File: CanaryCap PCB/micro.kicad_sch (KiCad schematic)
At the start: 36 parts, among them SW1 SW_MEC_5E, SW2 SW_MEC_5E, SW4 SW_MEC_5E, U3 ESP32-C6FH4

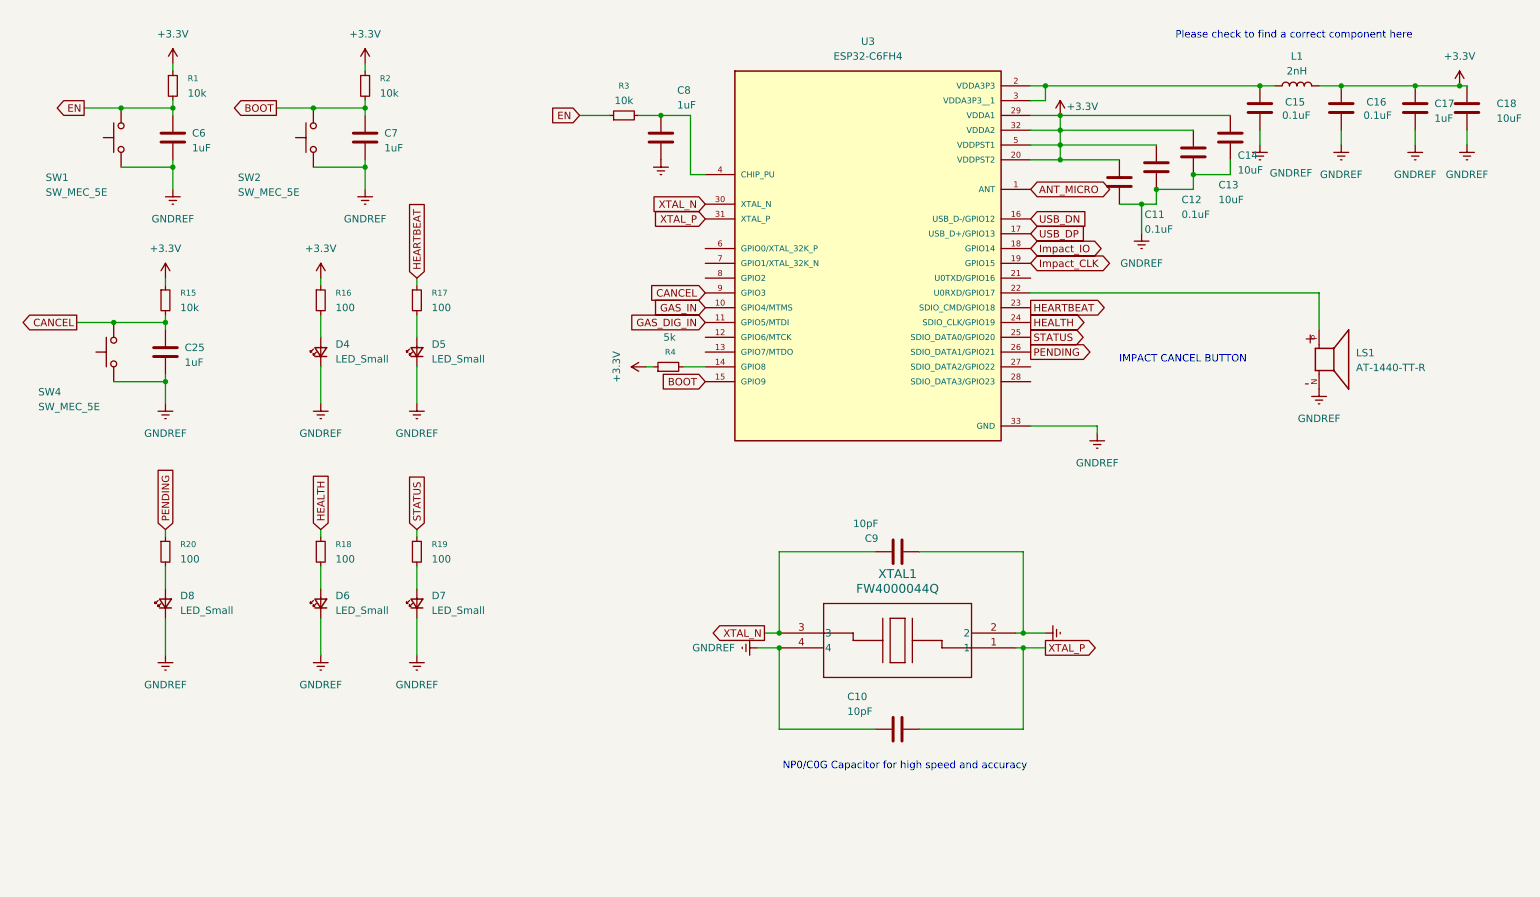
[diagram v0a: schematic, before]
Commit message: YIPPEE
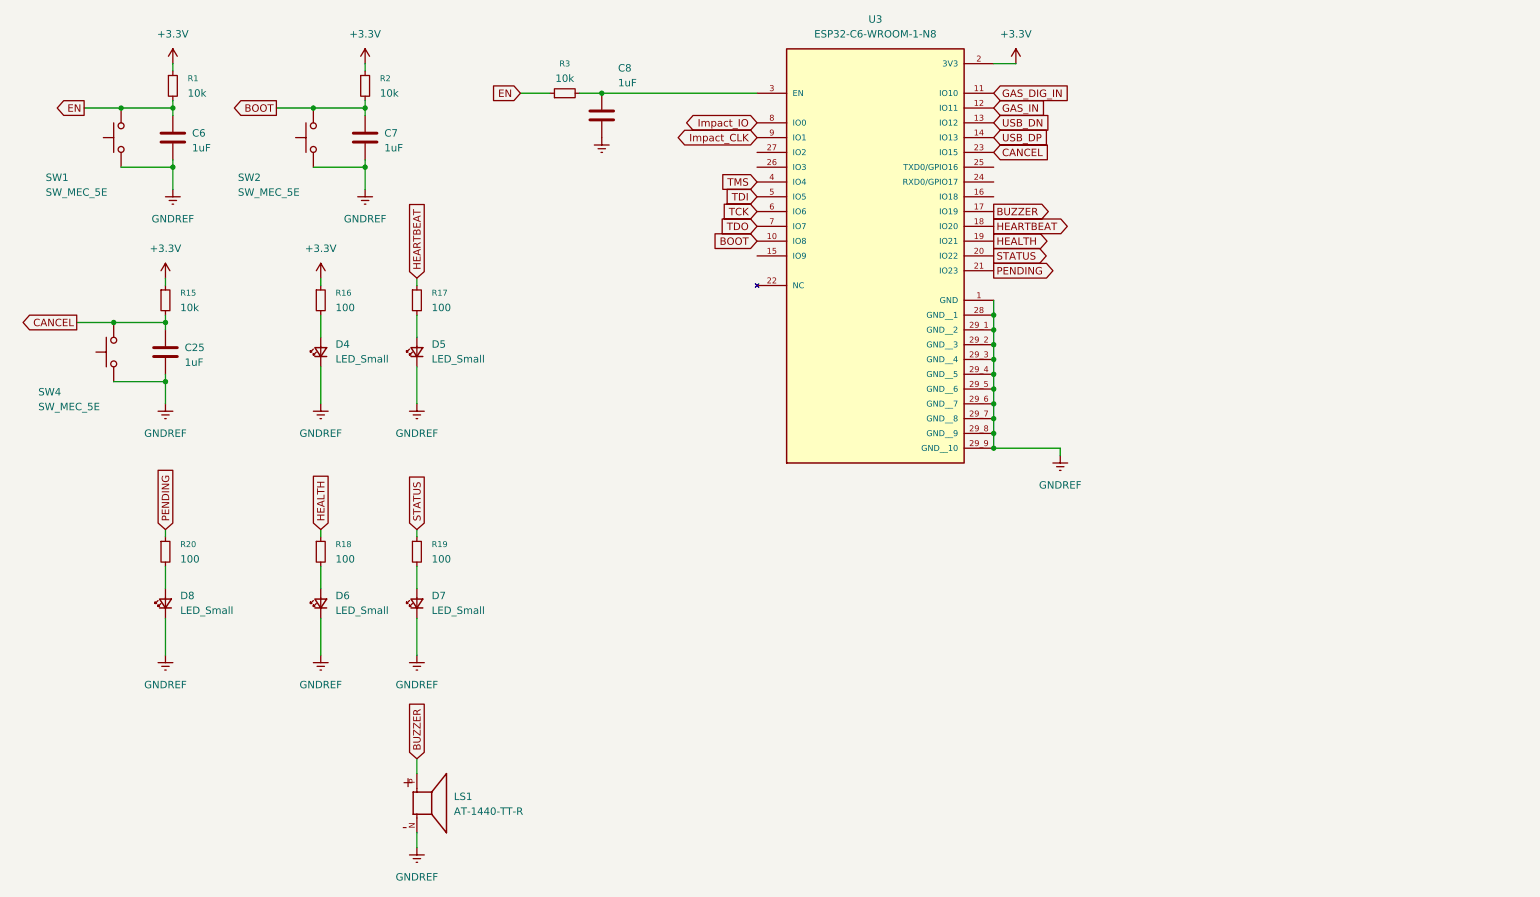
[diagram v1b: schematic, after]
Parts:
- removed C10, C9: 10pF, Capacitor_SMD:C_0603_1608Metric_Pad1.08x0.95mm_HandSolder, symbol Device:C
- removed C11, C12, C15, C16: 0.1uF, Capacitor_SMD:C_0603_1608Metric_Pad1.08x0.95mm_HandSolder, symbol Device:C
- removed C13, C14, C18: 10uF, Capacitor_SMD:C_0603_1608Metric_Pad1.08x0.95mm_HandSolder, symbol Device:C
- removed C17: 1uF, Capacitor_SMD:C_0603_1608Metric_Pad1.08x0.95mm_HandSolder, symbol Device:C
- removed L1: 2nH, Inductor_SMD:L_0603_1608Metric, symbol Device:L
- removed LS1: AT-1440-TT-R, AT-1440-TT-R:XDCR_AT-1440-TT-R, symbol AT-1440-TT-R:AT-1440-TT-R
- removed R4: 5k, Resistor_SMD:R_0603_1608Metric_Pad0.98x0.95mm_HandSolder, symbol Device:R_Small
- removed U3: ESP32-C6FH4, Package_DFN_QFN:QFN-32-1EP_5x5mm_P0.5mm_EP3.7x3.7mm, symbol ESP-32-C6:ESP32-C6FH4
- removed XTAL1: FW4000044Q, CRYSTAL4_FW4000044Q_DIO, symbol ESP-32-C6:FW4000044Q
- added LS1: AT-1440-TT-R, Library:XDCR_AT-1440-TT-R, symbol ESP-32-C6:AT-1440-TT-R
- added U3: ESP32-C6-WROOM-1-N8, Library:XCVR_ESP32-C6-WROOM-1-N8, symbol ESP-32-C6:ESP32-C6-WROOM-1-N8
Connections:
- net +3.3V: now also U3.2 (3V3)
- net BOOT: now also U3.10 (IO8)
- net CANCEL: now also U3.23 (IO15)
- net GAS_DIG_IN: now also U3.11 (IO10)
- net GAS_IN: now also U3.12 (IO11)
- net GNDREF: now also LS1.N, U3.1 (GND), U3.28 (GND__1), U3.29_1 (GND__2), U3.29_2 (GND__3), U3.29_3 (GND__4), U3.29_4 (GND__5), U3.29_5 (GND__6), U3.29_6 (GND__7), U3.29_7 (GND__8), U3.29_8 (GND__9), U3.29_9 (GND__10)
- net HEALTH: now also U3.19 (IO21)
- net HEARTBEAT: now also U3.18 (IO20)
- net Impact_CLK: now also U3.9 (IO1)
- net Impact_IO: now also U3.8 (IO0)
- net PENDING: now also U3.21 (IO23)
- net STATUS: now also U3.20 (IO22)
- net USB_DN: now also U3.13 (IO12)
- net USB_DP: now also U3.14 (IO13)
- net at C8.1, R3.2: now also U3.3 (EN)
- new net BUZZER: LS1.P, U3.17 (IO19)
- new net TCK: U3.6 (IO6)
- new net TDI: U3.5 (IO5)
- new net TDO: U3.7 (IO7)
- new net TMS: U3.4 (IO4)
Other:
- note removed: "IMPACT CANCEL BUTTON"
- note removed: "NP0/C0G Capacitor for high speed and accuracy"
- note removed: "Please check to find a correct component here"
- moved on the sheet: C8, R3

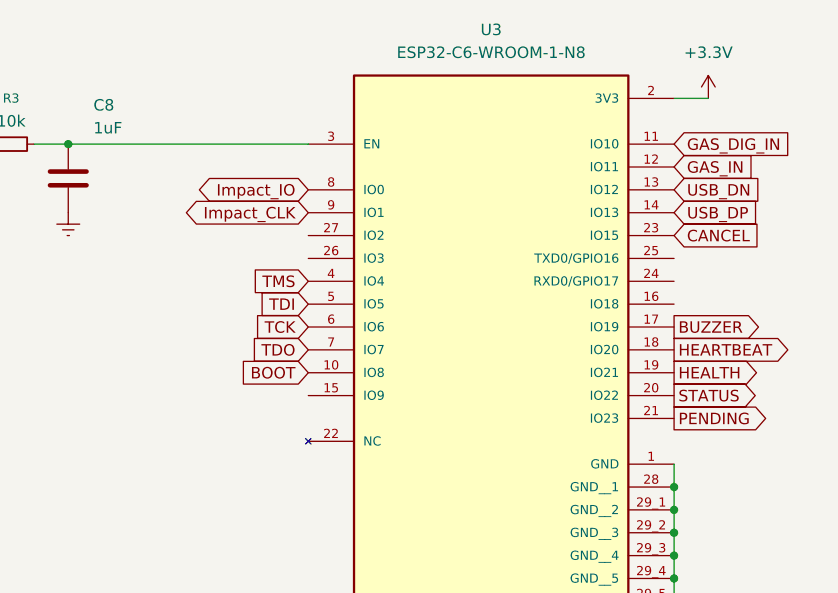
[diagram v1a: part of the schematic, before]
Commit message: Capcb updates
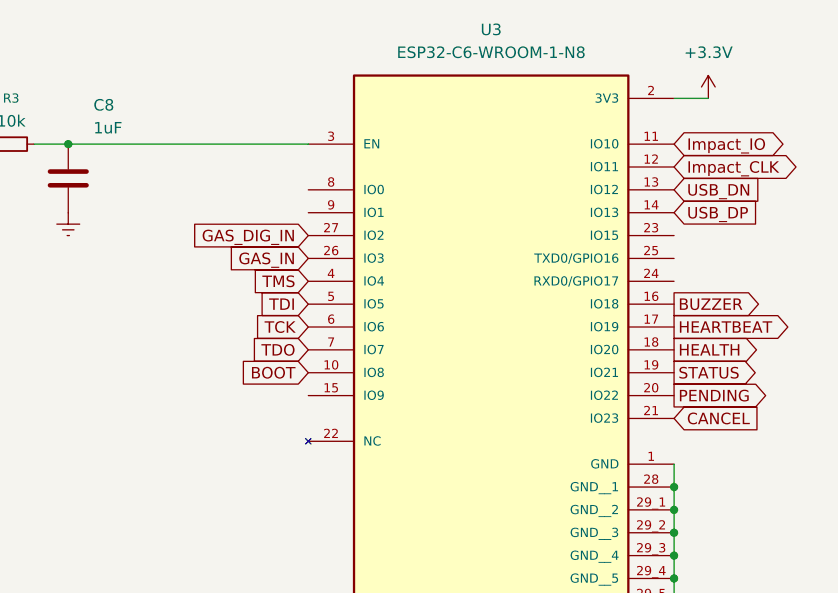
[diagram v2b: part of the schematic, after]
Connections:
- net BUZZER: now also U3.16 (IO18); no longer U3.17 (IO19)
- net CANCEL: now also U3.21 (IO23); no longer U3.23 (IO15)
- net GAS_DIG_IN: now also U3.27 (IO2); no longer U3.11 (IO10)
- net GAS_IN: now also U3.26 (IO3); no longer U3.12 (IO11)
- net HEALTH: now also U3.18 (IO20); no longer U3.19 (IO21)
- net HEARTBEAT: now also U3.17 (IO19); no longer U3.18 (IO20)
- net Impact_CLK: now also U3.12 (IO11); no longer U3.9 (IO1)
- net Impact_IO: now also U3.11 (IO10); no longer U3.8 (IO0)
- net PENDING: now also U3.20 (IO22); no longer U3.21 (IO23)
- net STATUS: now also U3.19 (IO21); no longer U3.20 (IO22)
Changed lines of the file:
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@@
 	(global_label "BUZZER"
 		(shape output)
-		(at 190.5 62.23 0)
-		(fields_autoplaced yes)
-		(effects
-			(font
-				(size 1.27 1.27)
-			)
-			(justify left)
-		)
-		(property "Intersheetrefs" "${INTERSHEET_REFS}"
-			(at 200.9237 62.23 0)
+		(at 190.5 59.69 0)
+		(fields_autoplaced yes)
+		(effects
+			(font
+				(size 1.27 1.27)
+			)
+			(justify left)
+		)
+		(property "Intersheetrefs" "${INTERSHEET_REFS}"
+			(at 200.9237 59.69 0)
 			(effects
 				(font
@@
 	(global_label "PENDING"
 		(shape output)
-		(at 190.5 72.39 0)
-		(fields_autoplaced yes)
-		(effects
-			(font
-				(size 1.27 1.27)
-			)
-			(justify left)
-		)
-		(property "Intersheetrefs" "${INTERSHEET_REFS}"
-			(at 201.71 72.39 0)
+		(at 190.5 69.85 0)
+		(fields_autoplaced yes)
+		(effects
+			(font
+				(size 1.27 1.27)
+			)
+			(justify left)
+		)
+		(property "Intersheetrefs" "${INTERSHEET_REFS}"
+			(at 201.71 69.85 0)
 			(effects
 				(font
@@
 	(global_label "Impact_CLK"
 		(shape bidirectional)
-		(at 149.86 49.53 180)
-		(fields_autoplaced yes)
-		(effects
-			(font
-				(size 1.27 1.27)
-			)
-			(justify right)
-		)
-		(property "Intersheetrefs" "${INTERSHEET_REFS}"
-			(at 134.8174 49.53 0)
-			(effects
-				(font
-					(size 1.27 1.27)
-				)
-				(justify right)
+		(at 190.5 44.45 0)
+		(fields_autoplaced yes)
+		(effects
+			(font
+				(size 1.27 1.27)
+			)
+			(justify left)
+		)
+		(property "Intersheetrefs" "${INTERSHEET_REFS}"
+			(at 205.5426 44.45 0)
+			(effects
+				(font
+					(size 1.27 1.27)
+				)
+				(justify left)
 				(hide yes)
 			)
@@
 	(global_label "HEALTH"
 		(shape output)
-		(at 190.5 67.31 0)
-		(fields_autoplaced yes)
-		(effects
-			(font
-				(size 1.27 1.27)
-			)
-			(justify left)
-		)
-		(property "Intersheetrefs" "${INTERSHEET_REFS}"
-			(at 200.3795 67.31 0)
+		(at 190.5 64.77 0)
+		(fields_autoplaced yes)
+		(effects
+			(font
+				(size 1.27 1.27)
+			)
+			(justify left)
+		)
+		(property "Intersheetrefs" "${INTERSHEET_REFS}"
+			(at 200.3795 64.77 0)
 			(effects
 				(font
@@
 	(global_label "GAS_IN"
 		(shape input)
-		(at 190.5 44.45 0)
-		(fields_autoplaced yes)
-		(effects
-			(font
-				(size 1.27 1.27)
-			)
-			(justify left)
-		)
-		(property "Intersheetrefs" "${INTERSHEET_REFS}"
-			(at 199.9562 44.45 0)
-			(effects
-				(font
-					(size 1.27 1.27)
-				)
-				(justify left)
+		(at 149.86 54.61 180)
+		(fields_autoplaced yes)
+		(effects
+			(font
+				(size 1.27 1.27)
+			)
+			(justify right)
+		)
+		(property "Intersheetrefs" "${INTERSHEET_REFS}"
+			(at 140.4038 54.61 0)
+			(effects
+				(font
+					(size 1.27 1.27)
+				)
+				(justify right)
 				(hide yes)
 			)
@@
 	(global_label "GAS_DIG_IN"
 		(shape input)
-		(at 190.5 41.91 0)
-		(fields_autoplaced yes)
-		(effects
-			(font
-				(size 1.27 1.27)
-			)
-			(justify left)
-		)
-		(property "Intersheetrefs" "${INTERSHEET_REFS}"
-			(at 204.0686 41.91 0)
-			(effects
-				(font
-					(size 1.27 1.27)
-				)
-				(justify left)
+		(at 149.86 52.07 180)
+		(fields_autoplaced yes)
+		(effects
+			(font
+				(size 1.27 1.27)
+			)
+			(justify right)
+		)
+		(property "Intersheetrefs" "${INTERSHEET_REFS}"
+			(at 136.2914 52.07 0)
+			(effects
+				(font
+					(size 1.27 1.27)
+				)
+				(justify right)
 				(hide yes)
 			)
@@
 	(global_label "CANCEL"
 		(shape input)
-		(at 190.5 52.07 0)
-		(fields_autoplaced yes)
-		(effects
-			(font
-				(size 1.27 1.27)
-			)
-			(justify left)
-		)
-		(property "Intersheetrefs" "${INTERSHEET_REFS}"
-			(at 200.6214 52.07 0)
+		(at 190.5 72.39 0)
+		(fields_autoplaced yes)
+		(effects
+			(font
+				(size 1.27 1.27)
+			)
+			(justify left)
+		)
+		(property "Intersheetrefs" "${INTERSHEET_REFS}"
+			(at 200.6214 72.39 0)
 			(effects
 				(font
@@
 	(global_label "Impact_IO"
 		(shape bidirectional)
-		(at 149.86 46.99 180)
-		(fields_autoplaced yes)
-		(effects
-			(font
-				(size 1.27 1.27)
-			)
-			(justify right)
-		)
-		(property "Intersheetrefs" "${INTERSHEET_REFS}"
-			(at 136.4502 46.99 0)
-			(effects
-				(font
-					(size 1.27 1.27)
-				)
-				(justify right)
+		(at 190.5 41.91 0)
+		(fields_autoplaced yes)
+		(effects
+			(font
+				(size 1.27 1.27)
+			)
+			(justify left)
+		)
+		(property "Intersheetrefs" "${INTERSHEET_REFS}"
+			(at 203.9098 41.91 0)
+			(effects
+				(font
+					(size 1.27 1.27)
+				)
+				(justify left)
 				(hide yes)
 			)
@@
 	(global_label "HEARTBEAT"
 		(shape output)
-		(at 190.5 64.77 0)
-		(fields_autoplaced yes)
-		(effects
-			(font
-				(size 1.27 1.27)
-			)
-			(justify left)
-		)
-		(property "Intersheetrefs" "${INTERSHEET_REFS}"
-			(at 203.7661 64.77 0)
+		(at 190.5 62.23 0)
+		(fields_autoplaced yes)
+		(effects
+			(font
+				(size 1.27 1.27)
+			)
+			(justify left)
+		)
+		(property "Intersheetrefs" "${INTERSHEET_REFS}"
+			(at 203.7661 62.23 0)
 			(effects
 				(font
@@
 	(global_label "STATUS"
 		(shape output)
-		(at 190.5 69.85 0)
-		(fields_autoplaced yes)
-		(effects
-			(font
-				(size 1.27 1.27)
-			)
-			(justify left)
-		)
-		(property "Intersheetrefs" "${INTERSHEET_REFS}"
-			(at 200.2585 69.85 0)
-			(effects
-				(font
+		(at 190.5 67.31 0)
+		(fields_autoplaced yes)
+		(effects
+			(font
+				(size 1.27 1.27)
+			)
+			(justify left)
+		)
+		(property "Intersheetrefs" "${INTERSHEET_REFS}"
+			(at 200.2585 67.31 0)
+			(effects
+				(font
